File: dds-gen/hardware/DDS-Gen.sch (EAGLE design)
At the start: 36 parts, among them IC1 TL072P, J1 POWER, J2 AVR_SPI_PROG_3X2PTH, J3 I2C CTRL, J4 BNCPTH, Q1 30MHz, U1 ATMEGA328P-PU

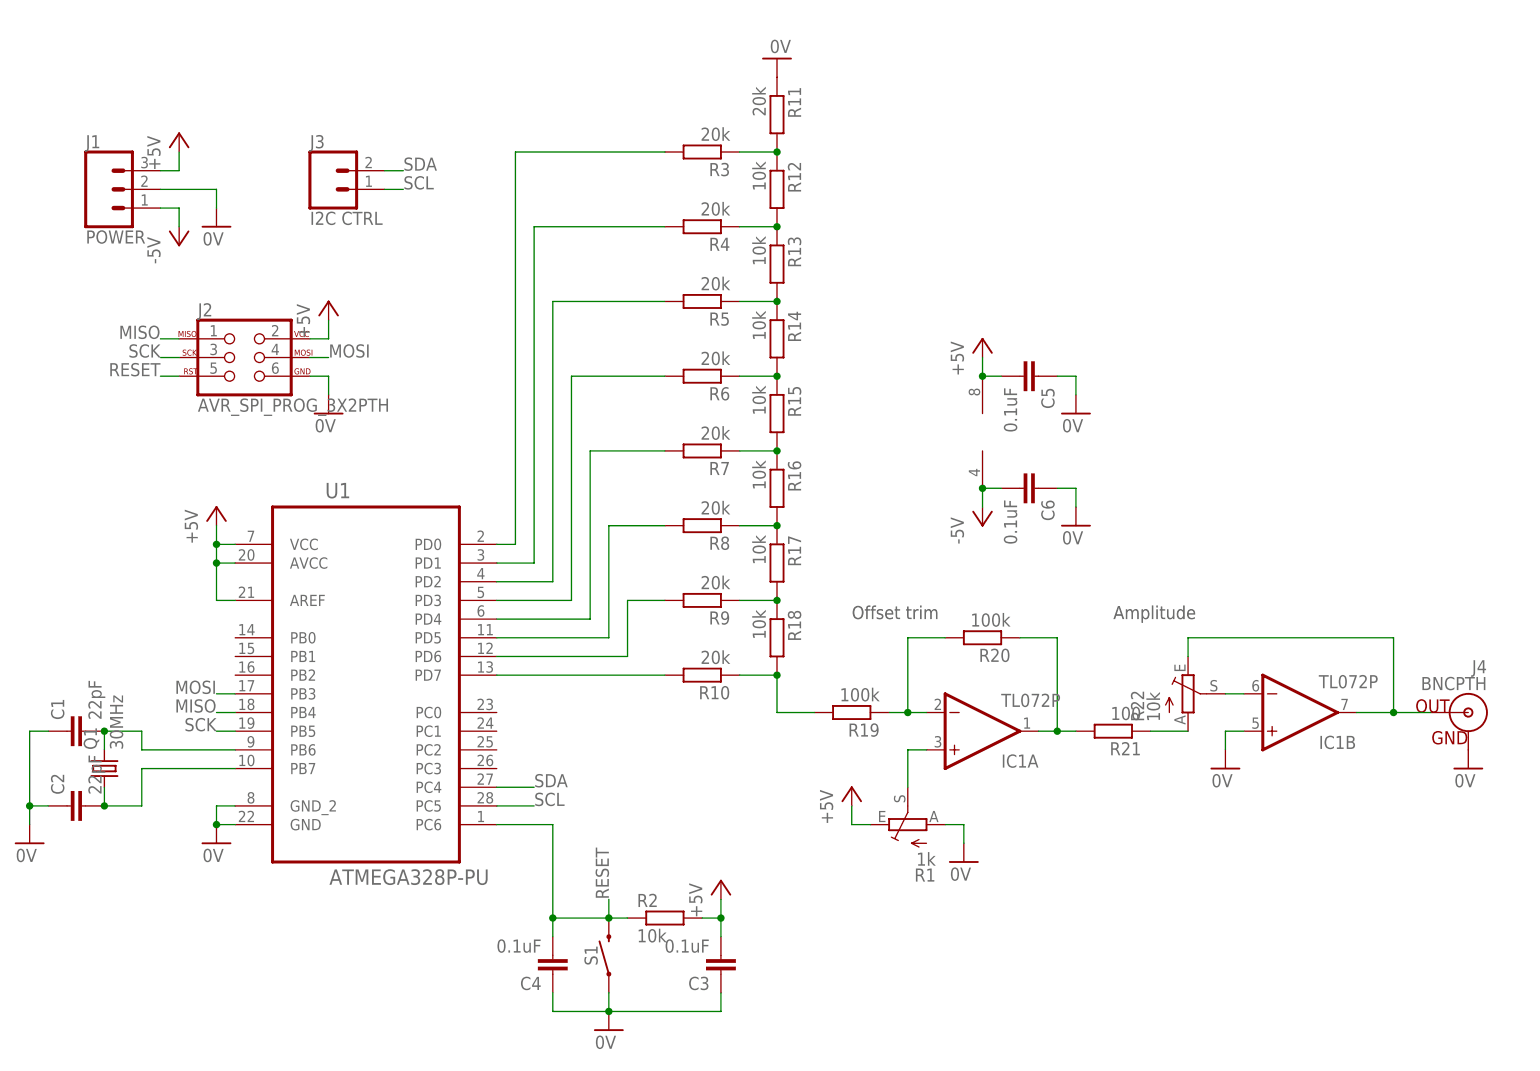
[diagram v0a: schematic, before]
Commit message: Updates begin layout of board, switched to ganged resistors
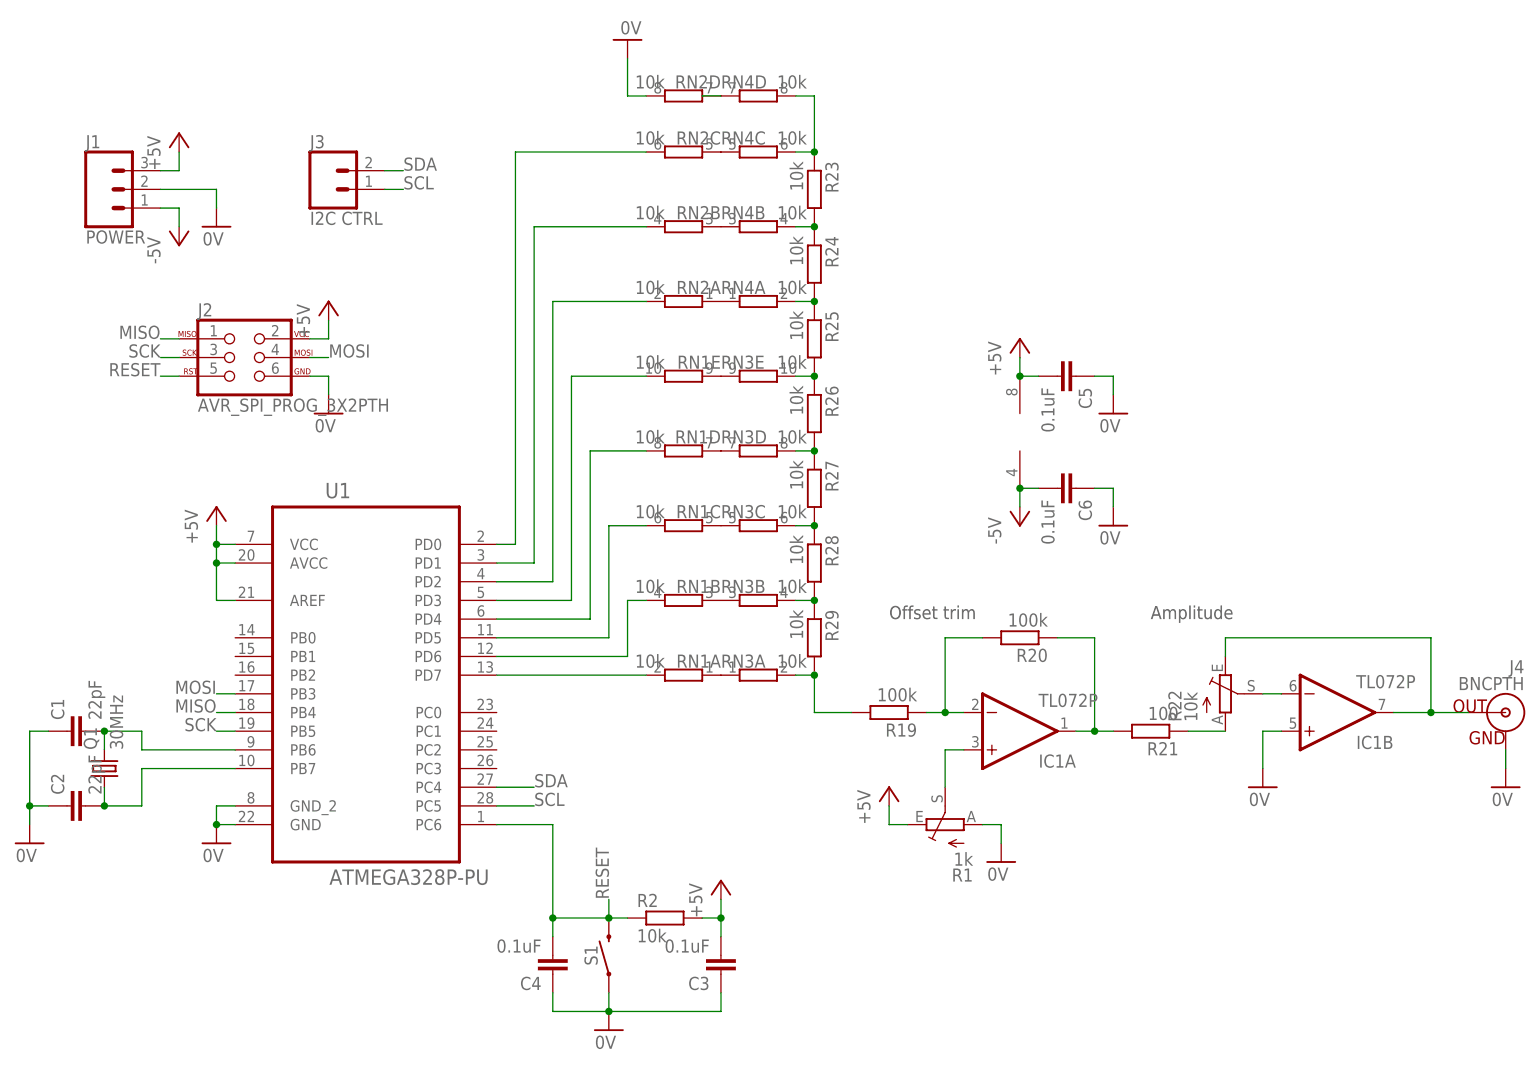
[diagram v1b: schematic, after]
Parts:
- removed R10, R11, R3, R4, R5, R6, R7, R8, R9: 20k, rcl:R-EU_0204/5
- removed R12, R13, R14, R15, R16, R17, R18: 10k, rcl:R-EU_0204/5
- added R23, R24, R25, R26, R27, R28, R29: 10k, rcl:R-EU_0204/5
- added RN1, RN2, RN3, RN4: 10k, resistor-sil:E5R
- R21: device rcl:R-EU_0204/5 -> resistor:R-EU_0204/7
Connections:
- removed net N$13: R17.2, R18.1, R9.1
- removed net N$14: R16.2, R17.1, R8.1
- removed net N$15: R15.2, R16.1, R7.1
- removed net N$16: R14.2, R15.1, R6.1
- removed net N$17: R13.2, R14.1, R5.1
- removed net N$18: R12.2, R13.1, R4.1
- removed net N$19: R11.2, R12.1, R3.1
- removed net N$20: R10.1, R18.2, R19.2
- new net N$25: RN1A.1, RN3A.1
- new net N$26: RN1B.1, RN3B.1
- new net N$27: RN1C.1, RN3C.1
- new net N$28: RN1D.1, RN3D.1
- new net N$29: RN1E.1, RN3E.1
- new net N$30: RN2A.1, RN4A.1
- new net N$31: RN2B.1, RN4B.1
- new net N$32: RN2C.1, RN4C.1
- new net N$33: RN2D.1, RN4D.1
- new net N$34: R23.1, RN4C.2, RN4D.2
- new net N$35: R23.2, R24.1, RN4B.2
- new net N$36: R24.2, R25.1, RN4A.2
- new net N$37: R25.2, R26.1, RN3E.2
- new net N$38: R26.2, R27.1, RN3D.2
- new net N$39: R27.2, R28.1, RN3C.2
- new net N$40: R28.2, R29.1, RN3B.2
- new net N$41: R19.2, R29.2, RN3A.2
- net 0V: now also RN2D.2; no longer R11.1
- net N$10: now also RN2A.2, U1.PD2; no longer R8.2, U1.PD5
- net N$11: now also RN2B.2, U1.PD1; no longer R9.2, U1.PD6
- net N$12: now also RN2C.2, U1.PD0; no longer R10.2, U1.PD7
- net N$5: now also RN1A.2, U1.PD7; no longer R3.2, U1.PD0
- net N$6: now also RN1B.2, U1.PD6; no longer R4.2, U1.PD1
- net N$7: now also RN1C.2, U1.PD5; no longer R5.2, U1.PD2
- net N$8: now also RN1D.2, U1.PD4; no longer R6.2, U1.PD3
- net N$9: now also RN1E.2, U1.PD3; no longer R7.2, U1.PD4
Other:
- moved on the sheet: C5, C6, IC1A, IC1B, J4, R1, R19, R20, R21, R22
